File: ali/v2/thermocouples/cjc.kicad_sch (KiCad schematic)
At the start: 23 parts, among them U10 TMP117AIDRVR, U11 TMP117AIDRVR, U12 TMP117AIDRVR, U13 TMP117AIDRVR, U7 TCA9543A, U8 TMP117AIDRVR, U9 TMP117AIDRVR

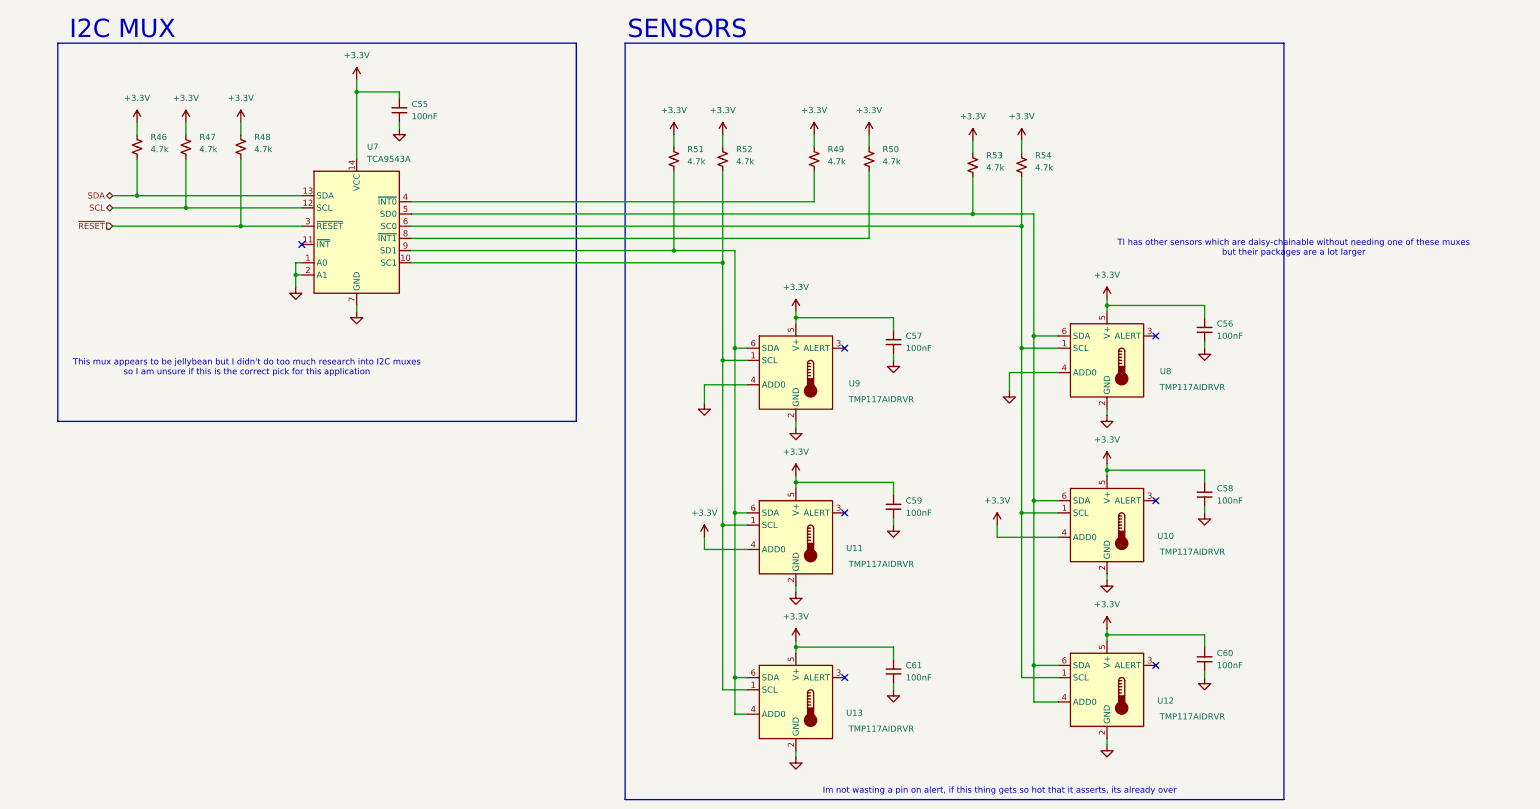
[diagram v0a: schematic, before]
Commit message: Begin prep for second board review
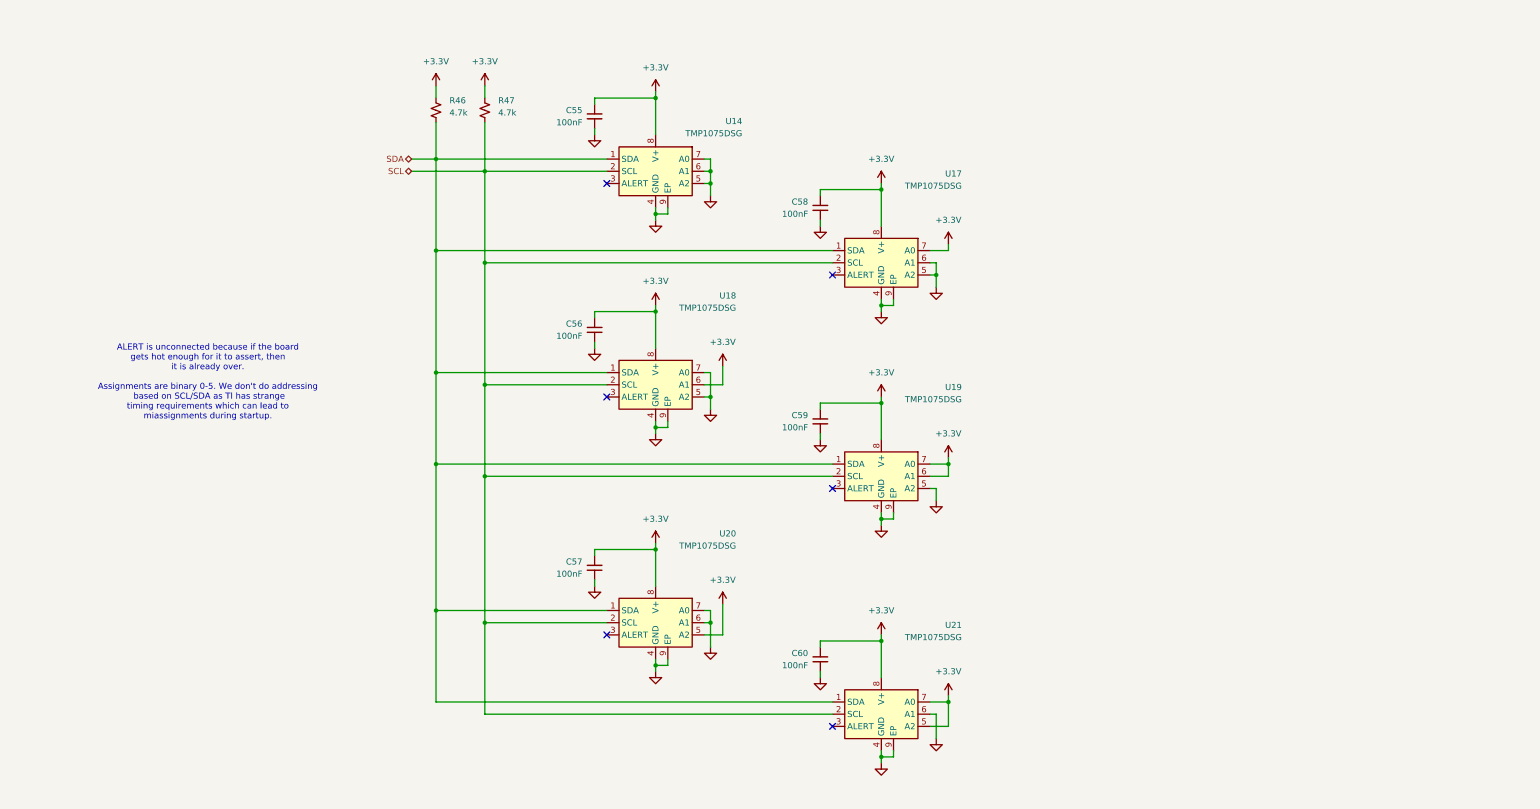
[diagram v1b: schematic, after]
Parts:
- removed C61: 100nF, APRL_Passive:C_0603, symbol Device:C_Small
- removed R48, R49, R50, R51, R52, R53, R54: 4.7k, APRL_Passive:R_0603, symbol Device:R_Small_US
- removed U10, U11, U12, U13, U8, U9: TMP117AIDRVR, Package_SON:WSON-6-1EP_2x2mm_P0.65mm_EP1x1.6mm, symbol APRL_Analog:TMP117xxDRV
- removed U7: TCA9543A, APRL_Package:TSSOP-14_4.4x5mm_P0.65mm, symbol APRL_Comms:TCA9543A
- added U14, U17, U18, U19, U20, U21: TMP1075DSG, Package_SON:Texas_DSG0008A_WSON-8-1EP_2x2mm_P0.5mm_EP0.9x1.6mm_ThermalVias, symbol Sensor_Temperature:TMP1075DSG
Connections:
- net +3.3V: now also U14.8 (V+), U17.7 (A0), U17.8 (V+), U18.6 (A1), U18.8 (V+), U19.6 (A1), U19.7 (A0), U19.8 (V+), U20.5 (A2), U20.8 (V+), U21.5 (A2), U21.7 (A0), U21.8 (V+)
- net GND: now also U14.4 (GND), U14.5 (A2), U14.6 (A1), U14.7 (A0), U14.9 (EP), U17.4 (GND), U17.5 (A2), U17.6 (A1), U17.9 (EP), U18.4 (GND), U18.5 (A2), U18.7 (A0), U18.9 (EP), U19.4 (GND), U19.5 (A2), U19.9 (EP), U20.4 (GND), U20.6 (A1), U20.7 (A0), U20.9 (EP), U21.4 (GND), U21.6 (A1), U21.9 (EP)
- net SCL: now also U14.2 (SCL), U17.2 (SCL), U18.2 (SCL), U19.2 (SCL), U20.2 (SCL), U21.2 (SCL)
- net SDA: now also U14.1 (SDA), U17.1 (SDA), U18.1 (SDA), U19.1 (SDA), U20.1 (SDA), U21.1 (SDA)
- no-connect marks 7 -> 6
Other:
- note added: "ALERT is unconnected because if the board gets hot enough for it to assert, then it is already over. Assignments are binary 0-5. We don't do addressing based on SCL/SDA as TI has strange timing requirements which can lead to miassignments during startup."
- note removed: "I2C MUX"
- note removed: "Im not wasting a pin on alert, if this thing gets so hot that it asserts, its already over"
- note removed: "SENSORS"
- note removed: "TI has other sensors which are daisy-chainable without needing one of these muxes but their packages are a lot larger"
- note removed: "This mux appears to be jellybean but I didn't do too much research into I2C muxes so I am unsure if this is the correct pick for this application"
- moved on the sheet: R46, R47
